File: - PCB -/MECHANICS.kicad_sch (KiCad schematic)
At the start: 7 parts, among them SW1 SW_SPDT, SW3 SW_Push

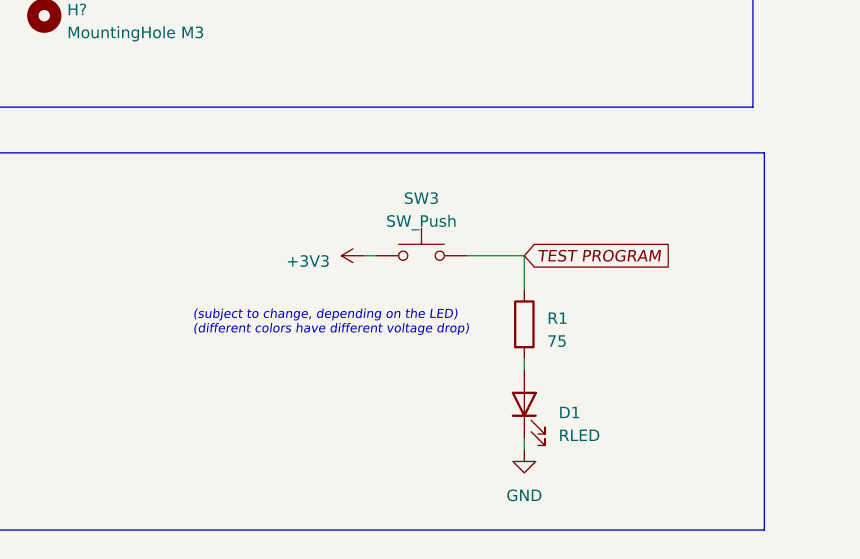
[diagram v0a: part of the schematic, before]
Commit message: Board update
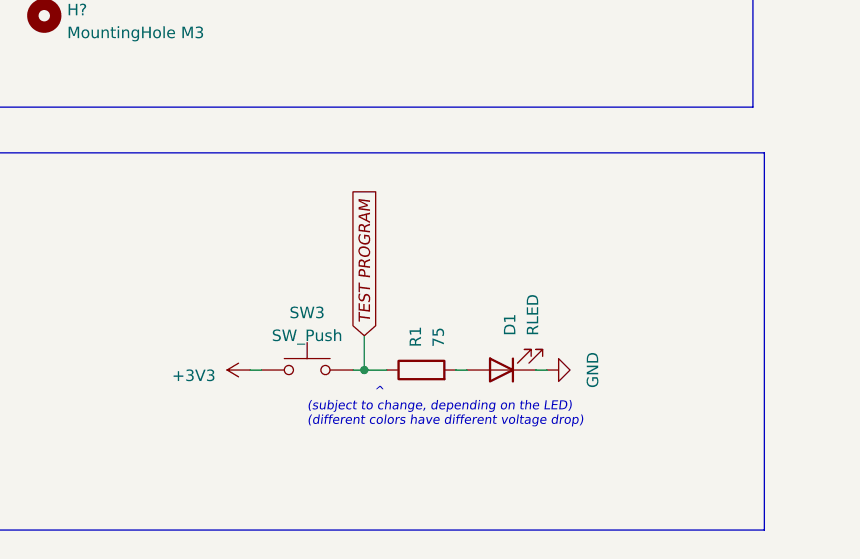
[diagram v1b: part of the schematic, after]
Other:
- note added: "^ (subject to change, depending on the LED) (different colors have different voltage drop)"
- note removed: "(subject to change, depending on the LED) (different colors have different voltage drop)"
- moved on the sheet: D1, R1, SW3
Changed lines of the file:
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@@
 (kicad_sch (version 20230121) (generator eeschema)
   (paper "A4")
+  (junction (at 173.99 139.7) (diameter 0) (color 0 0 0 0)
+  )
   (no_connect (at 97.79 97.79))
   (polyline (pts (xy 66.04 115.57) (xy 218.44 115.57))
     (stroke (width 0) (type default))
   )
-  (wire (pts (xy 191.77 147.32) (xy 191.77 148.59))
+  (wire (pts (xy 193.04 139.7) (xy 194.31 139.7))
     (stroke (width 0) (type default))
   )
@@
     (stroke (width 0) (type default))
   )
-  (wire (pts (xy 191.77 139.7) (xy 191.77 138.43))
-    (stroke (width 0) (type default))
-  )
-  (wire (pts (xy 191.77 127) (xy 191.77 130.81))
+  (wire (pts (xy 185.42 139.7) (xy 184.15 139.7))
     (stroke (width 0) (type default))
   )
@@
     (stroke (width 0) (type default))
   )
-  (wire (pts (xy 173.99 127) (xy 175.26 127))
+  (wire (pts (xy 161.29 139.7) (xy 162.56 139.7))
     (stroke (width 0) (type default))
   )
@@
     (stroke (width 0) (type default))
   )
-  (wire (pts (xy 191.77 127) (xy 185.42 127))
+  (wire (pts (xy 173.99 139.7) (xy 176.53 139.7))
+    (stroke (width 0) (type default))
+  )
+  (wire (pts (xy 172.72 139.7) (xy 173.99 139.7))
+    (stroke (width 0) (type default))
+  )
+  (wire (pts (xy 173.99 135.89) (xy 173.99 139.7))
     (stroke (width 0) (type default))
   )
@@
     (effects (font (size 1.27 1.27) italic) (justify left bottom))
   )
-  (text "(subject to change, depending on the LED)\n(different colors have different voltage drop)"
-    (at 154.94 135.89 0)
+  (text "                 ^\n(subject to change, depending on the LED)\n(different colors have different voltage drop)"
+    (at 167.64 146.05 0)
     (effects (font (size 1 1) italic) (justify left bottom))
   )
-  (global_label "TEST PROGRAM" (shape input) (at 191.77 127 0) (fields_autoplaced)
+  (global_label "TEST PROGRAM" (shape input) (at 173.99 135.89 90) (fields_autoplaced)
     (effects (font (size 1.27 1.27) italic) (justify left))
-    (property "Intersheetrefs" "${INTERSHEET_REFS}" (at 208.8045 127 0)
+    (property "Intersheetrefs" "${INTERSHEET_REFS}" (at 173.99 118.8555 90)
       (effects (font (size 1.27 1.27)) (justify left) hide)
     )
@@
     )
   )
-  (symbol (lib_id "power:GND") (at 191.77 148.59 0) (unit 1)
-    (in_bom yes) (on_board yes) (dnp no) (fields_autoplaced)
-    (property "Reference" "#PWR03" (at 191.77 154.94 0)
-      (effects (font (size 1.27 1.27)) hide)
-    )
-    (property "Value" "GND" (at 191.77 153.67 0)
-      (effects (font (size 1.27 1.27)))
-    )
-    (property "Footprint" "" (at 191.77 148.59 0)
-      (effects (font (size 1.27 1.27)) hide)
-    )
-    (property "Datasheet" "" (at 191.77 148.59 0)
+  (symbol (lib_id "power:GND") (at 194.31 139.7 90) (unit 1)
+    (in_bom yes) (on_board yes) (dnp no) (fields_autoplaced)
+    (property "Reference" "#PWR03" (at 200.66 139.7 0)
+      (effects (font (size 1.27 1.27)) hide)
+    )
+    (property "Value" "GND" (at 199.39 139.7 0)
+      (effects (font (size 1.27 1.27)))
+    )
+    (property "Footprint" "" (at 194.31 139.7 0)
+      (effects (font (size 1.27 1.27)) hide)
+    )
+    (property "Datasheet" "" (at 194.31 139.7 0)
       (effects (font (size 1.27 1.27)) hide)
     )
@@
     )
   )
-  (symbol (lib_id "Switch:SW_Push") (at 180.34 127 0) (unit 1)
-    (in_bom yes) (on_board yes) (dnp no) (fields_autoplaced)
-    (property "Reference" "SW3" (at 180.34 120.65 0)
-      (effects (font (size 1.27 1.27)))
-    )
-    (property "Value" "SW_Push" (at 180.34 123.19 0)
-      (effects (font (size 1.27 1.27)))
-    )
-    (property "Footprint" "Button_Switch_THT:SW_PUSH_6mm" (at 180.34 121.92 0)
-      (effects (font (size 1.27 1.27)) hide)
-    )
-    (property "Datasheet" "~" (at 180.34 121.92 0)
+  (symbol (lib_id "Switch:SW_Push") (at 167.64 139.7 0) (unit 1)
+    (in_bom yes) (on_board yes) (dnp no) (fields_autoplaced)
+    (property "Reference" "SW3" (at 167.64 133.35 0)
+      (effects (font (size 1.27 1.27)))
+    )
+    (property "Value" "SW_Push" (at 167.64 135.89 0)
+      (effects (font (size 1.27 1.27)))
+    )
+    (property "Footprint" "Button_Switch_THT:SW_PUSH_6mm" (at 167.64 134.62 0)
+      (effects (font (size 1.27 1.27)) hide)
+    )
+    (property "Datasheet" "~" (at 167.64 134.62 0)
       (effects (font (size 1.27 1.27)) hide)
     )
@@
     )
   )
-  (symbol (lib_id "power:+3V3") (at 173.99 127 90) (unit 1)
-    (in_bom yes) (on_board yes) (dnp no) (fields_autoplaced)
-    (property "Reference" "#PWR02" (at 177.8 127 0)
-      (effects (font (size 1.27 1.27)) hide)
-    )
-    (property "Value" "+3V3" (at 170.18 127.635 90)
-      (effects (font (size 1.27 1.27)) (justify left))
-    )
-    (property "Footprint" "" (at 173.99 127 0)
-      (effects (font (size 1.27 1.27)) hide)
-    )
-    (property "Datasheet" "" (at 173.99 127 0)
+  (symbol (lib_id "power:+3V3") (at 161.29 139.7 90) (unit 1)
+    (in_bom yes) (on_board yes) (dnp no) (fields_autoplaced)
+    (property "Reference" "#PWR02" (at 165.1 139.7 0)
+      (effects (font (size 1.27 1.27)) hide)
+    )
+    (property "Value" "+3V3" (at 157.48 140.335 90)
+      (effects (font (size 1.27 1.27)) (justify left))
+    )
+    (property "Footprint" "" (at 161.29 139.7 0)
+      (effects (font (size 1.27 1.27)) hide)
+    )
+    (property "Datasheet" "" (at 161.29 139.7 0)
       (effects (font (size 1.27 1.27)) hide)
     )
@@
     )
   )
-  (symbol (lib_id "Device:R") (at 191.77 134.62 0) (unit 1)
-    (in_bom yes) (on_board yes) (dnp no) (fields_autoplaced)
-    (property "Reference" "R1" (at 194.31 133.985 0)
-      (effects (font (size 1.27 1.27)) (justify left))
-    )
-    (property "Value" "75 " (at 194.31 136.525 0)
-      (effects (font (size 1.27 1.27)) (justify left))
-    )
-    (property "Footprint" "Resistor_THT:R_Axial_DIN0207_L6.3mm_D2.5mm_P10.16mm_Horizontal" (at 189.992 134.62 90)
-      (effects (font (size 1.27 1.27)) hide)
-    )
-    (property "Datasheet" "~" (at 191.77 134.62 0)
+  (symbol (lib_id "Device:R") (at 180.34 139.7 90) (unit 1)
+    (in_bom yes) (on_board yes) (dnp no) (fields_autoplaced)
+    (property "Reference" "R1" (at 179.705 137.16 0)
+      (effects (font (size 1.27 1.27)) (justify left))
+    )
+    (property "Value" "75 " (at 182.245 137.16 0)
+      (effects (font (size 1.27 1.27)) (justify left))
+    )
+    (property "Footprint" "Resistor_THT:R_Axial_DIN0207_L6.3mm_D2.5mm_P10.16mm_Horizontal" (at 180.34 141.478 90)
+      (effects (font (size 1.27 1.27)) hide)
+    )
+    (property "Datasheet" "~" (at 180.34 139.7 0)
       (effects (font (size 1.27 1.27)) hide)
     )
@@
     )
   )
-  (symbol (lib_id "Device:LED") (at 191.77 143.51 90) (unit 1)
-    (in_bom yes) (on_board yes) (dnp no) (fields_autoplaced)
-    (property "Reference" "D1" (at 195.58 144.4625 90)
+  (symbol (lib_id "Device:LED") (at 189.23 139.7 180) (unit 1)
+    (in_bom yes) (on_board yes) (dnp no) (fields_autoplaced)
+    (property "Reference" "D1" (at 190.1825 135.89 90)
       (effects (font (size 1.27 1.27)) (justify right))
     )
-    (property "Value" "RLED" (at 195.58 147.0025 90)
+    (property "Value" "RLED" (at 192.7225 135.89 90)
       (effects (font (size 1.27 1.27)) (justify right))
     )
-    (property "Footprint" "LED_THT:LED_D5.0mm" (at 191.77 143.51 0)
-      (effects (font (size 1.27 1.27)) hide)
-    )
-    (property "Datasheet" "~" (at 191.77 143.51 0)
-      (effects (font (size 1.27 1.27)) hide)
-    )
+    (property "Footprint" "LED_THT:LED_D5.0mm" (at 189.23 139.7 0)
+      (effects (font (size 1.27 1.27)) hide)
+    )
+    (property "Datasheet" "~" (at 189.23 139.7 0)
+      (effects (font (size 1.27 1.27)) hide)
+    )
